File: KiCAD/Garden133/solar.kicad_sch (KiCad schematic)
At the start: 16 parts, among them Q1 FS8205A, Q2 AO3401A, U5 DW01A, U6 TP4056

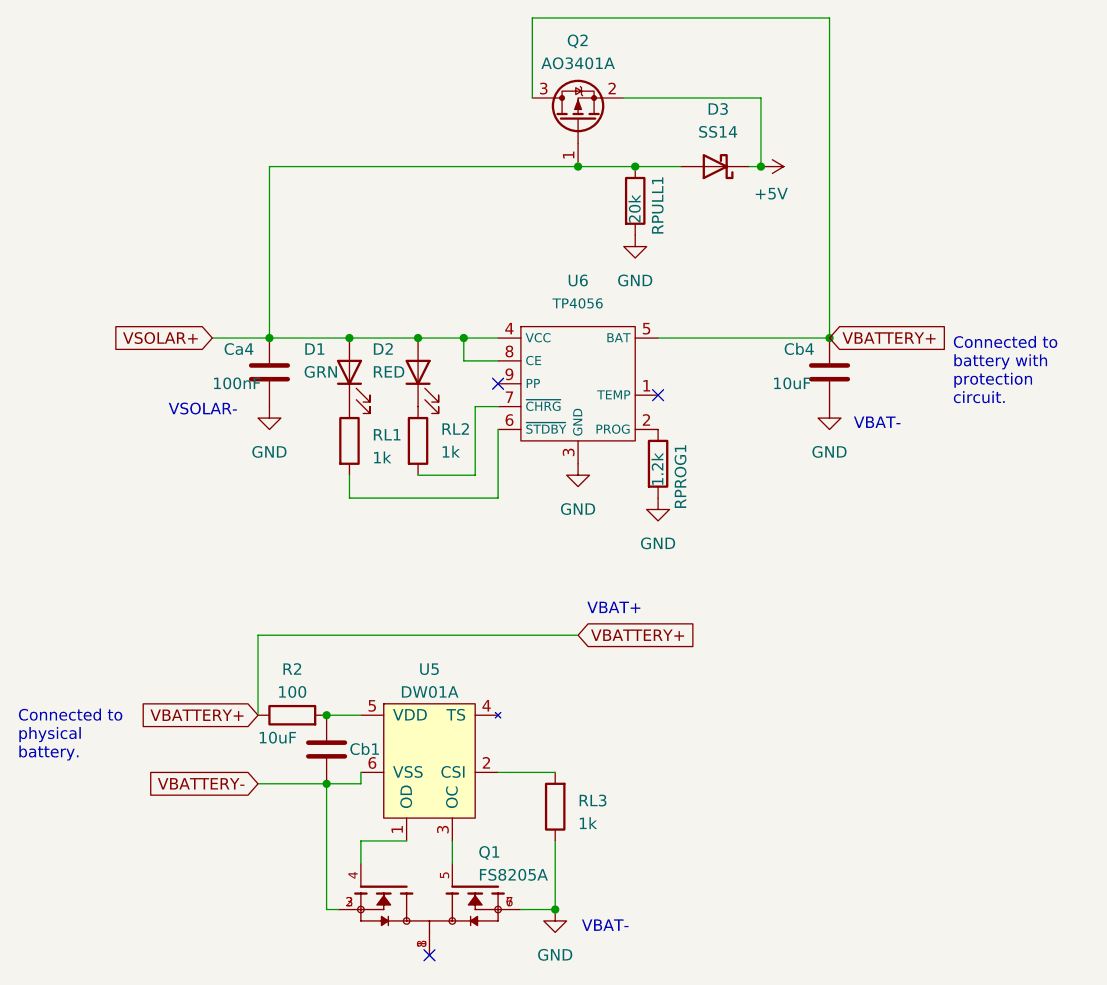
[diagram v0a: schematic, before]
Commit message: Board version 5
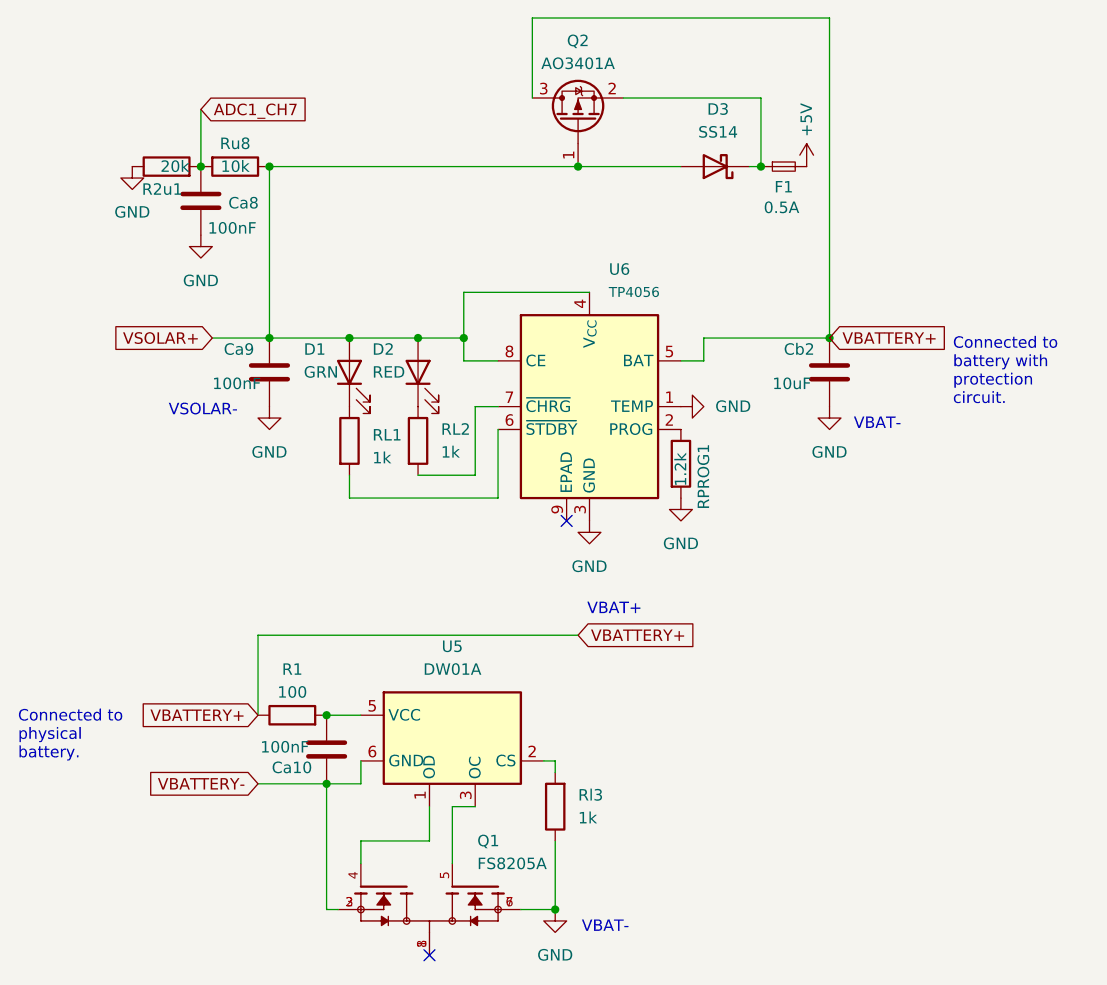
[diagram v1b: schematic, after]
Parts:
- added Ca8: 100nF, Capacitor_SMD:C_0603_1608Metric_Pad1.08x0.95mm_HandSolder, symbol Device:C
- added F1: 0.5A, Diode_SMD:D_0805_2012Metric, symbol Device:Fuse_Small
- added Ru8: 10k, Resistor_SMD:R_0603_1608Metric, symbol Device:R
- Ca10: renamed from Cb1; value 10uF -> 100nF; footprint Capacitor_SMD:C_0805_2012Metric_Pad1.18x1.45mm_HandSolder -> Capacitor_SMD:C_0603_1608Metric_Pad1.08x0.95mm_HandSolder
- U5: symbol marbastlib-various:DW01A -> Battery_Management:DW01A
- U6: footprint Package_SO:SOIC-8-1EP_3.9x4.9mm_P1.27mm_EP2.29x3mm -> Package_SO:SOIC-8-1EP_3.9x4.9mm_P1.27mm_EP2.41x3.3mm_ThermalVias; symbol TP4056:TP4056 -> Battery_Management:TP4056-42-ESOP8
- renumbered Ca4 to Ca9, Cb4 to Cb2, R2 to R1, RPULL1 to R2u1, RL3 to Rl3
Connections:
- net +5V: now also F1.2; no longer D3.1 (K), Q2.2 (S)
- net GND: now also R2u1.1, U6.1 (TEMP), Ca8.1; no longer R2u1.2
- net VSOLAR+: now also Ru8.1; no longer R2u1.1
- new net: D3.1 (K), F1.1, Q2.2 (S)
- new net ADC1_CH7: Ca8.2, R2u1.2, Ru8.2
- no-connect marks 3 -> 2
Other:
- moved on the sheet: R2u1, RPROG1
